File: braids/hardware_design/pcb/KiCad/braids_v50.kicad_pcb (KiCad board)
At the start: 2 copper layers, 78.7 x 106.7 mm, 120 parts, among them IC1 74595D, IC10 TL072, IC2 74595D, IC3 LM4040B25, IC4 MCP3204, IC5 DAC8551, IC6 LM1117-3.3, IC7 MCP6004, IC8 LM4040B10, IC9 TL074D, J1 PJ301_THONKICONN6, J2 PJ301_THONKICONN6, J3 PJ301_THONKICONN6, J4 PJ301_THONKICONN6, J5 PJ301_THONKICONN6, J6 PJ301_THONKICONN6, Q1 MMBT3904, Q2 MMBT3904, Q3 MMBT3904, Q4 MMBT3904, Q5 8MHz, Q6 MMBT3904, SW1 EC12E_SW, SW2 EVQQ2, SW3 EVQQ2

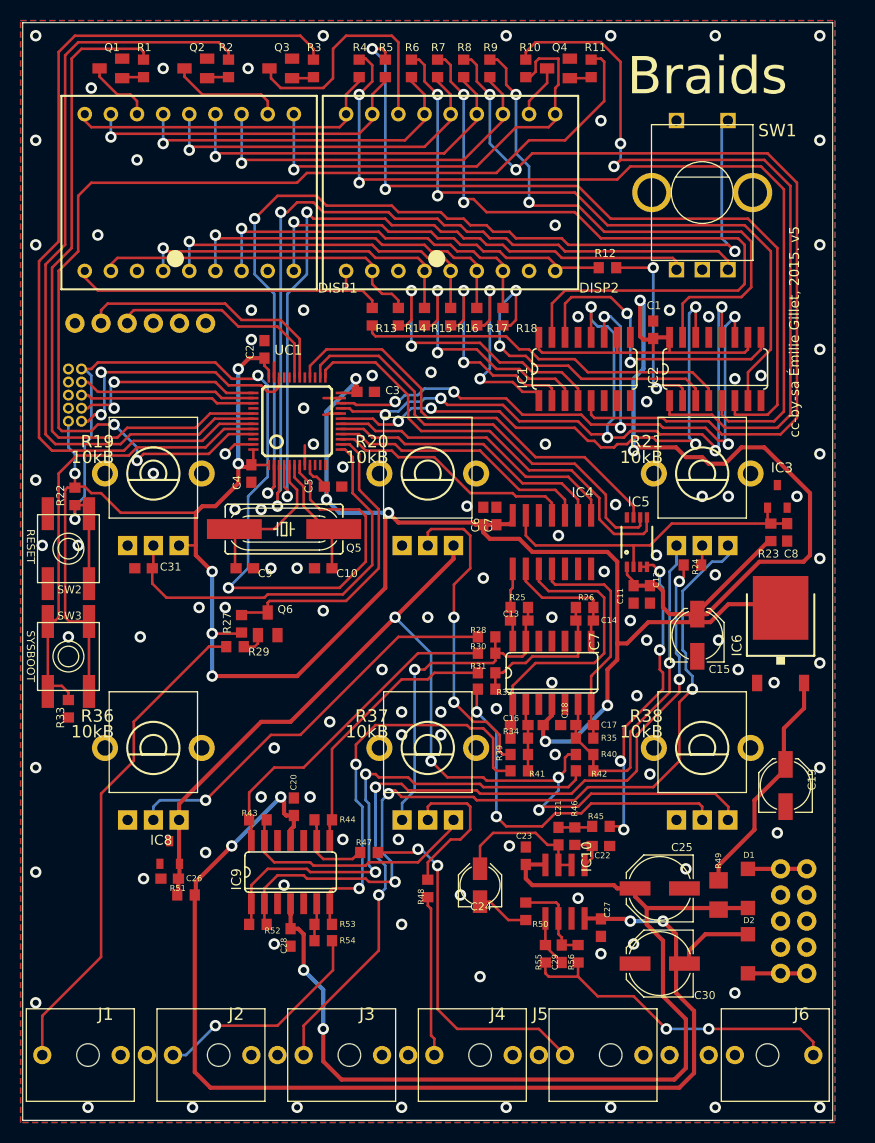
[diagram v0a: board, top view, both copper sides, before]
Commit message: clouds import etc.
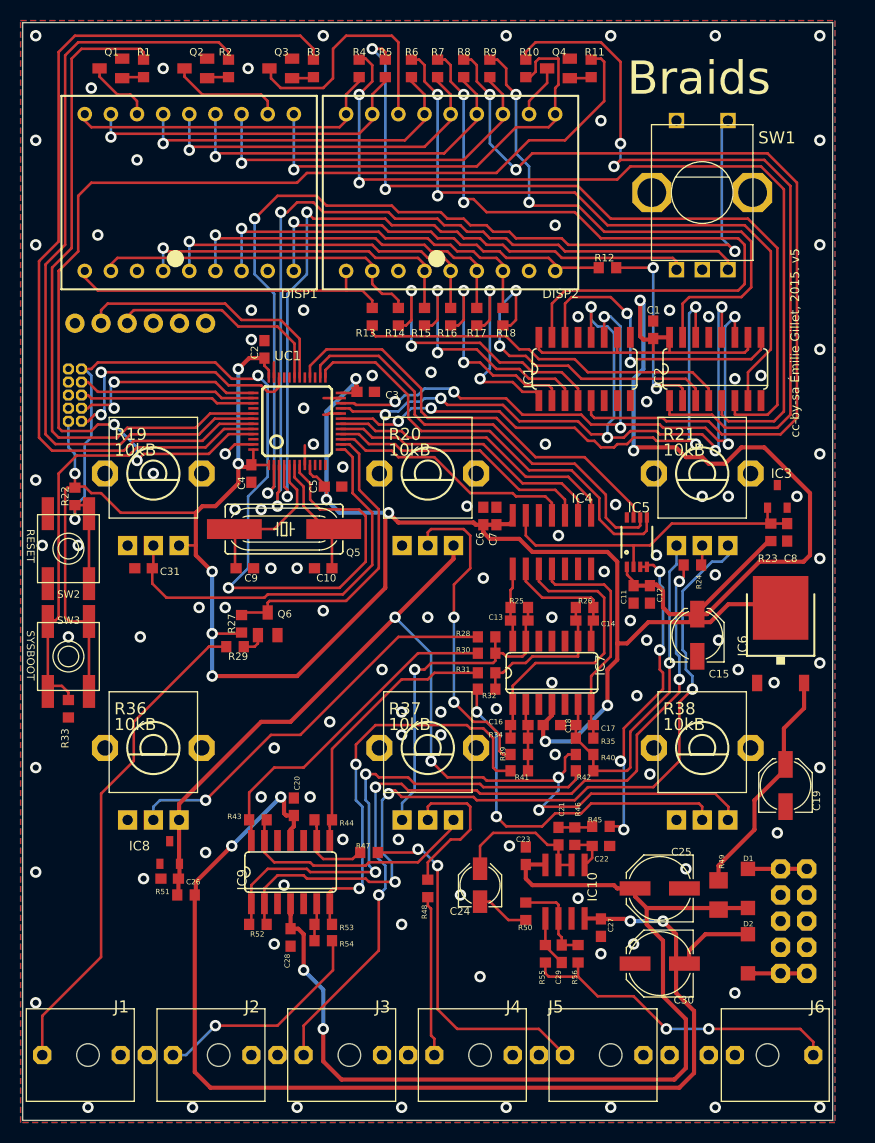
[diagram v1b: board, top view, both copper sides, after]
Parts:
- IC1, IC2: value 74595D -> 74HC595D
- JP3: value M06SIP -> (none)
- SW2, SW3: value EVQQ2 -> (none)
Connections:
- net /braids_v50_1/ADC_MISO renamed ADC_MISO
- net /braids_v50_1/ADC_MOSI renamed ADC_MOSI
- net /braids_v50_1/ADC_SCK renamed ADC_SCK
- net /braids_v50_1/ADC_SS renamed ADC_SS
- net /braids_v50_1/BOOT_FLASH renamed BOOT_FLASH
- net /braids_v50_1/DAC_MOSI renamed DAC_MOSI
- net /braids_v50_1/DAC_SCK renamed DAC_SCK
- net /braids_v50_1/DAC_SS renamed DAC_SS
- net /braids_v50_1/DISP_CHAR0 renamed DISP_CHAR0
- net /braids_v50_1/DISP_CHAR1 renamed DISP_CHAR1
- net /braids_v50_1/DISP_CHAR2 renamed DISP_CHAR2
- net /braids_v50_1/DISP_CHAR3 renamed DISP_CHAR3
- net /braids_v50_1/DISP_EN renamed DISP_EN
- net /braids_v50_1/DISP_SCK renamed DISP_SCK
- net /braids_v50_1/DISP_SER renamed DISP_SER
- net /braids_v50_1/ENC_A renamed ENC_A
- net /braids_v50_1/ENC_B renamed ENC_B
- net /braids_v50_1/ENC_CLICK renamed ENC_CLICK
- net /braids_v50_1/FINE_TUNE renamed FINE_TUNE
- net /braids_v50_1/JTCK renamed JTCK
- net /braids_v50_1/JTDI renamed JTDI
- net /braids_v50_1/JTDO renamed JTDO
- net /braids_v50_1/JTMS renamed JTMS
- net /braids_v50_1/RESET renamed RESET
- net /braids_v50_1/RX renamed RX
- net /braids_v50_1/TX renamed TX
- DISP1 pad 8: Net-(DISP1-Pad8) -> (no net)
- DISP2 pad 8: Net-(DISP2-Pad8) -> (no net)
- IC1 pad 6: Net-(IC1-Pad6) -> (no net)
- IC1 pad 7: Net-(IC1-Pad7) -> (no net)
- IC1 pad 9: Net-(IC1-Pad9) -> (no net)
- J1 pad P2: Net-(J1-PadP2) -> (no net)
- J2 pad P2: Net-(J2-PadP2) -> (no net)
- J3 pad P2: Net-(J3-PadP2) -> (no net)
- J4 pad P2: Net-(J4-PadP2) -> (no net)
- J5 pad P2: Net-(J5-PadP2) -> (no net)
- J6 pad P2: Net-(J6-PadP2) -> (no net)
- JP2 pad 7: Net-(JP2-Pad7) -> (no net)
- JP3 pad 2: Net-(JP3-Pad2) -> (no net)
- JP3 pad 3: Net-(JP3-Pad3) -> (no net)
- JP3 pad 6: Net-(JP3-Pad6) -> (no net)
- UC1 pad 10: Net-(UC1-Pad10) -> (no net)
- UC1 pad 11: Net-(UC1-Pad11) -> (no net)
- UC1 pad 12: Net-(UC1-Pad12) -> (no net)
- UC1 pad 27: Net-(UC1-Pad27) -> (no net)
- UC1 pad 29: Net-(UC1-Pad29) -> (no net)
- UC1 pad 32: Net-(UC1-Pad32) -> (no net)
- UC1 pad 33: Net-(UC1-Pad33) -> (no net)
- UC1 pad 40: Net-(UC1-Pad40) -> (no net)
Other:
- net class Default removed
- rule pad_to_mask_clearance: 0.051 -> 0
